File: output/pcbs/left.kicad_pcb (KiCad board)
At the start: 2 copper layers, 123.6 x 92.5 mm, 19 parts

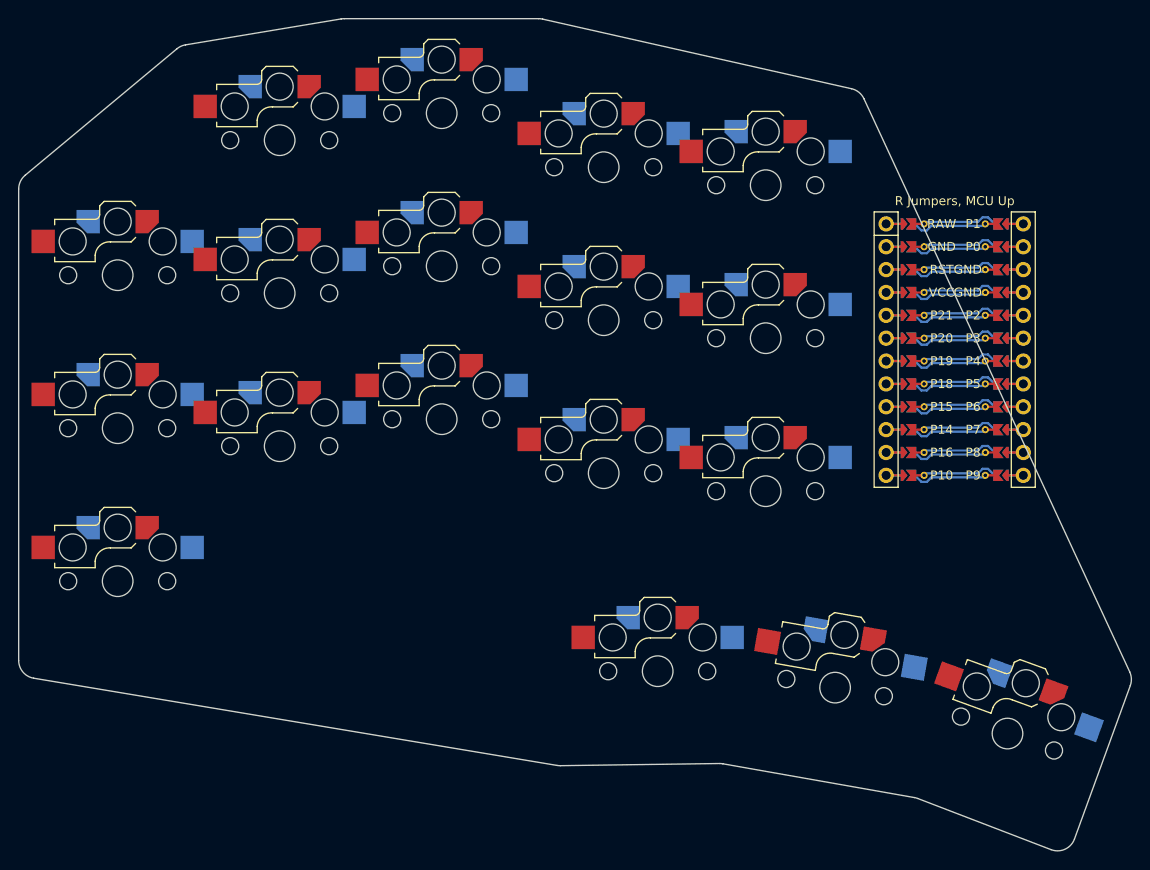
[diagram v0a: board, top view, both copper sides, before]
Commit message: More gentle tweaking
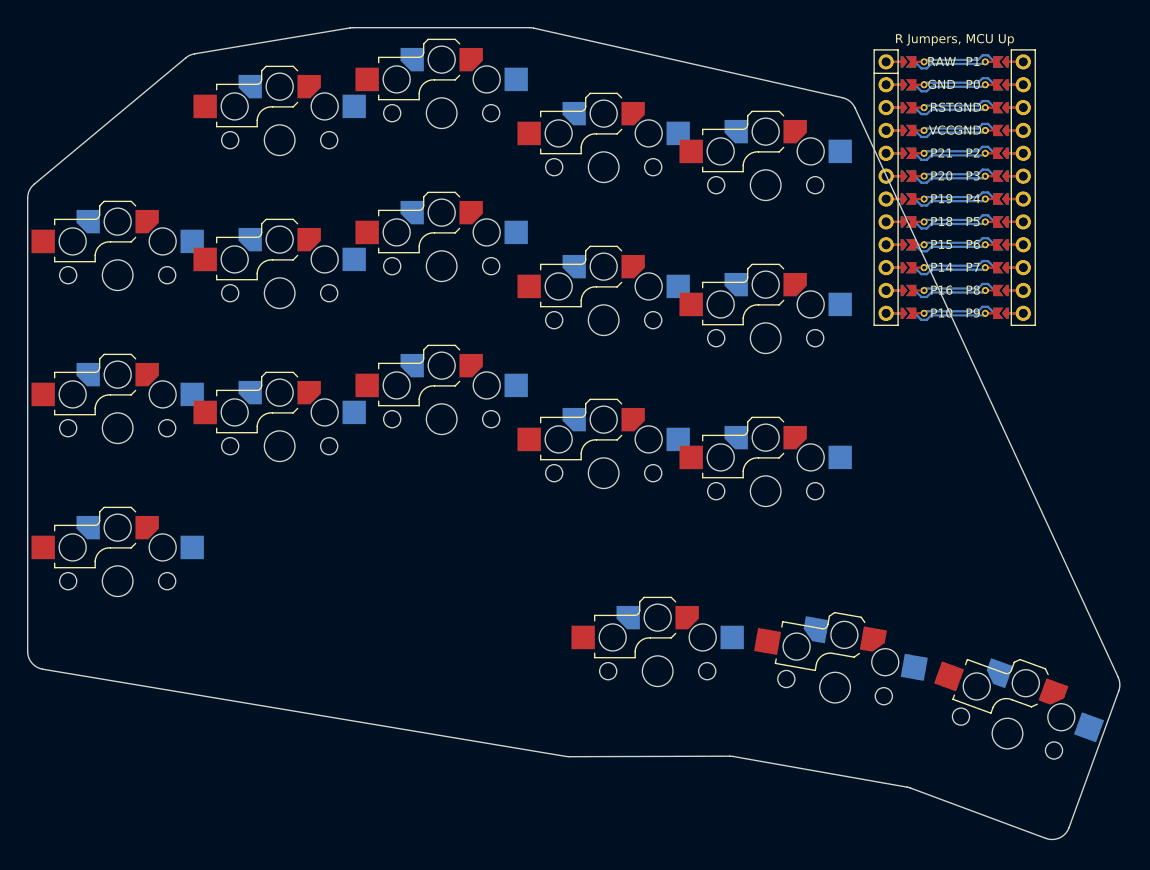
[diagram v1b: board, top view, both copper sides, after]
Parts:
- moved MCU1 18.0 mm to (93.0, -45.0)
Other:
- board size 123.6 x 92.5 mm -> 121.3 x 90.2 mm
